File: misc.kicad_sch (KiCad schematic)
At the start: 46 parts, among them J2 Tag-Connect_TC2030-IDC-NL_2x3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, U1 MPFS250T-FCVG484, U2 SDINBDG4-8G, U3 MT25QL01GBBB1EW9-0SIT

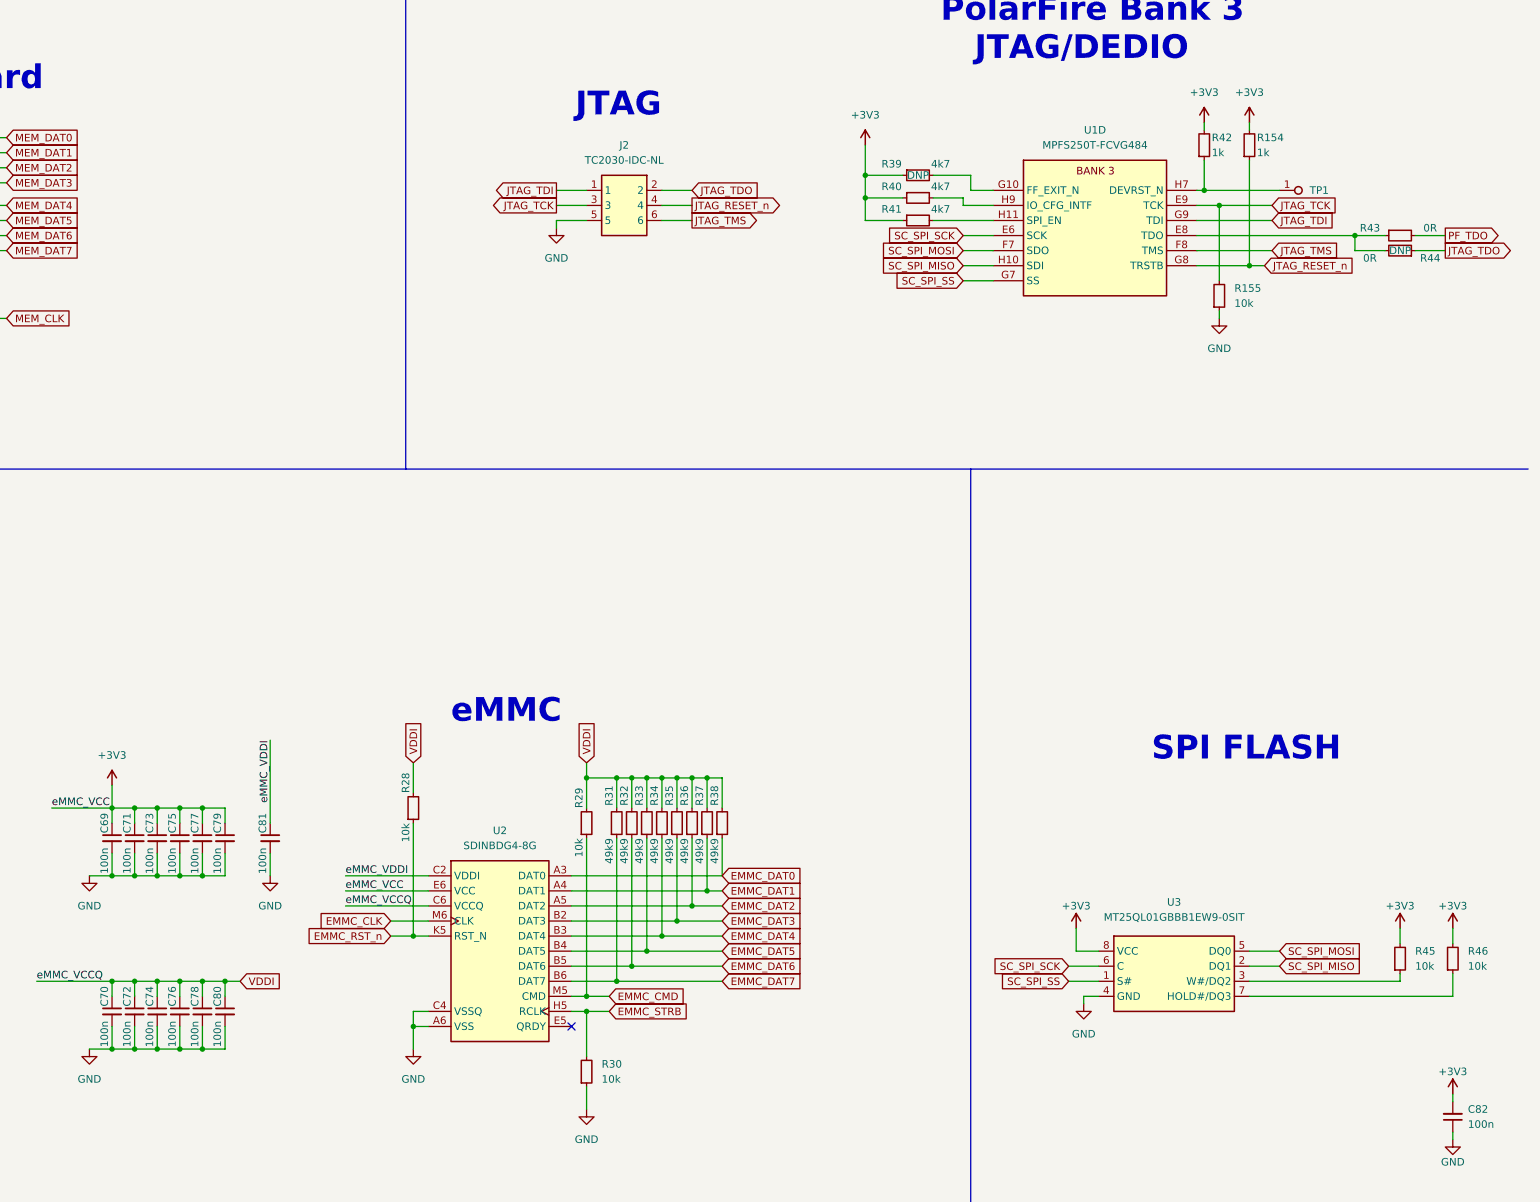
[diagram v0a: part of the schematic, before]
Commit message: [#54899] Update symbols
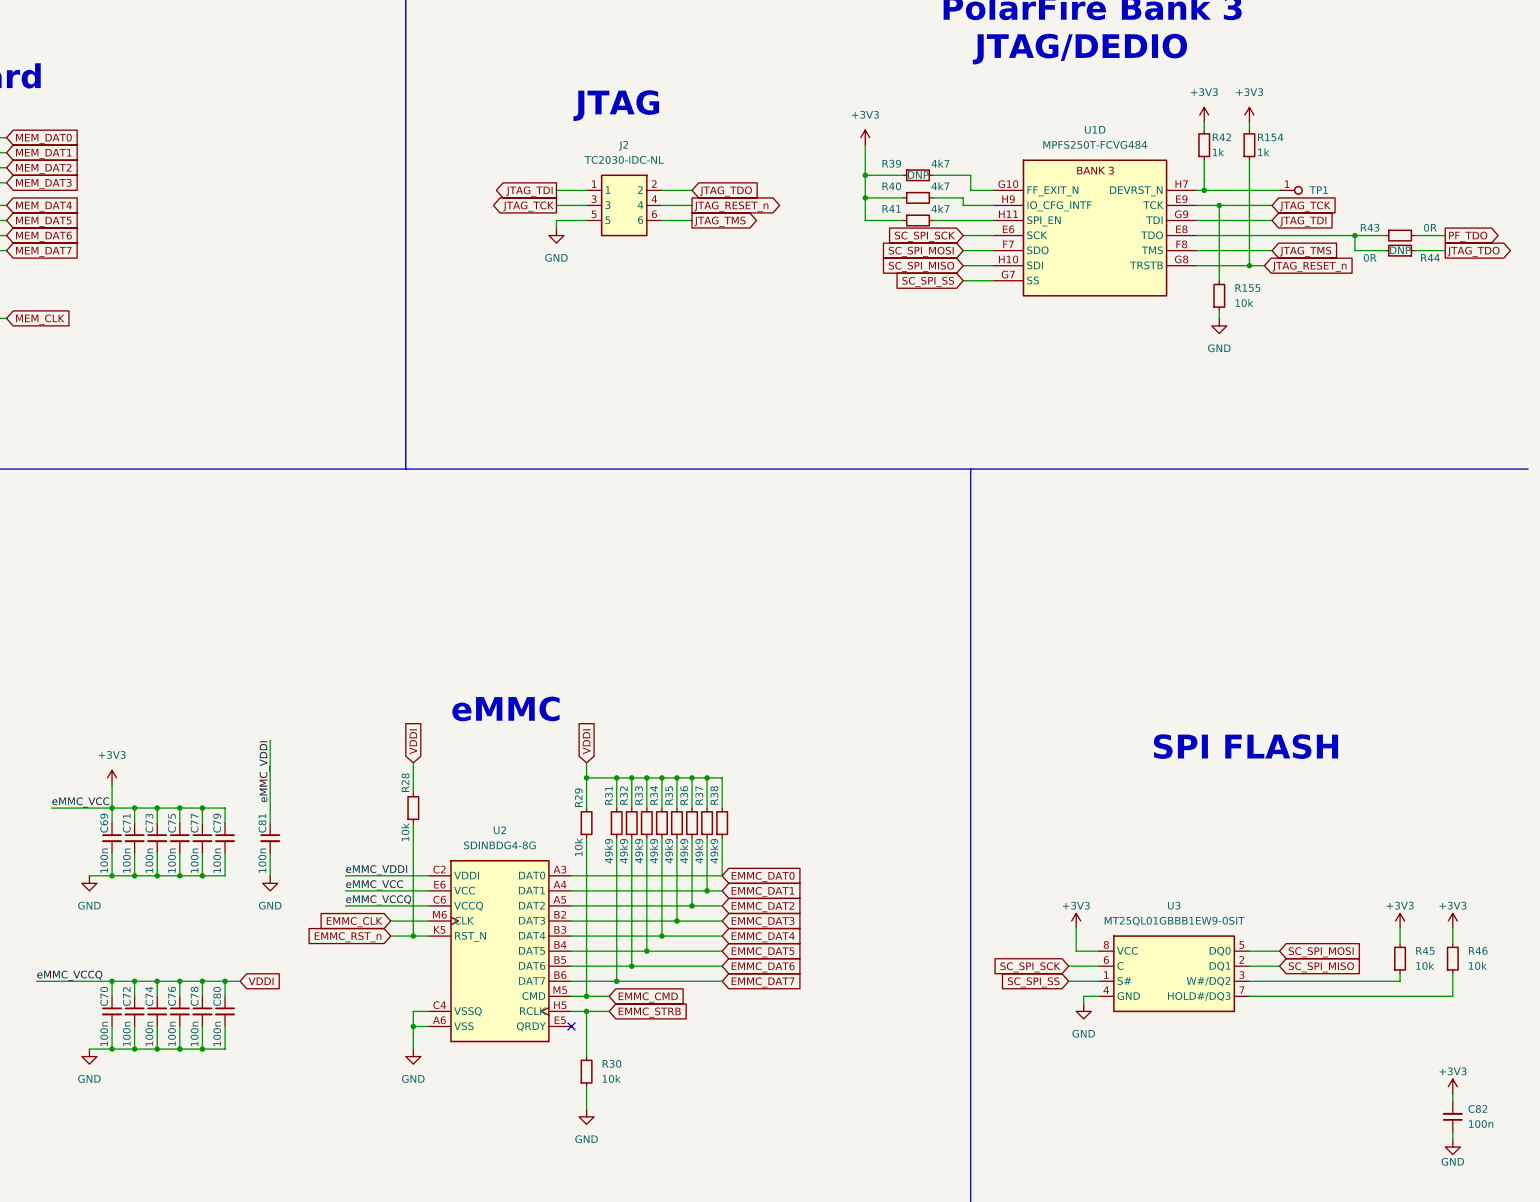
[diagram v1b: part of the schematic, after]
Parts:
- R25, R26, R27, R44: now in the parts list
- U1: footprint antmicro-footprints:BGA-484_19x19mm_Layout22x22_P0.8mm_FCVG484 -> antmicro-footprints:BGA-484_19x19mm_Layout22x22_P0.8mm_MPFS250T-FCVG484
- U3: value MT25QL01GBBB1EW9-0SIT -> MT25QL01GBBB1EW9-0SIT; symbol antmicroMemory:MT25QL01GBBB1EW9-0SIT -> antmicroMemory:MT25QL01GBBB1EW9-0SIT; MPN MT25QL01GBBB1EW9-0SIT -> MT25QL01GBBB1EW9-0SIT
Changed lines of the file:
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@@
   )
   (symbol (lib_id "antmicroResistorNetworksArrays:R_4x0R_0201_array") (at 138.43 66.04 0) (unit 1)
-    (in_bom no) (on_board yes) (dnp no)
+    (in_bom yes) (on_board yes) (dnp no)
     (property "Reference" "R25" (at 143.51 59.69 0)
       (effects (font (size 1.27 1.27) (thickness 0.15)))
@@
   )
   (symbol (lib_id "antmicroResistors0402:R_0R_0402") (at 388.62 85.09 180) (unit 1)
-    (in_bom no) (on_board yes) (dnp no)
+    (in_bom yes) (on_board yes) (dnp no)
     (property "Reference" "R44" (at 391.16 86.36 0)
       (effects (font (size 1.27 1.27) (thickness 0.15)))
@@
   )
   (symbol (lib_id "antmicroResistors0402:R_0R_0402") (at 140.97 96.52 0) (unit 1)
-    (in_bom no) (on_board yes) (dnp no)
+    (in_bom yes) (on_board yes) (dnp no)
     (property "Reference" "R27" (at 138.43 95.25 0)
       (effects (font (size 1.27 1.27) (thickness 0.15)))
@@
       (effects (font (size 1.27 1.27) (thickness 0.15)) (justify left bottom) hide)
     )
-    (property "Footprint" "antmicro-footprints:BGA-484_19x19mm_Layout22x22_P0.8mm_FCVG484" (at 157.48 208.28 0)
+    (property "Footprint" "antmicro-footprints:BGA-484_19x19mm_Layout22x22_P0.8mm_MPFS250T-FCVG484" (at 157.48 208.28 0)
       (effects (font (size 1.27 1.27) (thickness 0.15)) (justify left bottom) hide)
     )
@@
     )
   )
-  (symbol (lib_id "antmicroMemory:MT25QL01GBBB1EW9-0SIT ") (at 335.28 203.2 0) (unit 1)
+  (symbol (lib_id "antmicroMemory:MT25QL01GBBB1EW9-0SIT") (at 335.28 203.2 0) (unit 1)
     (in_bom yes) (on_board yes) (dnp no) (fields_autoplaced)
-    (property "Reference" "U3" (at 347.98 194.945 0)
-      (effects (font (size 1.27 1.27) (thickness 0.15)))
-    )
-    (property "Value" "MT25QL01GBBB1EW9-0SIT " (at 378.46 210.82 0)
+    (property "Reference" "U3" (at 347.98 195.58 0)
+      (effects (font (size 1.27 1.27) (thickness 0.15)))
+    )
+    (property "Value" "MT25QL01GBBB1EW9-0SIT" (at 378.46 210.82 0)
       (effects (font (size 1.27 1.27) (thickness 0.15)) (justify left bottom) hide)
     )
@@
       (effects (font (size 1.27 1.27) (thickness 0.15)) (justify left bottom) hide)
     )
-    (property "Datasheet" "https://www.mouser.pl/datasheet/2/671/mict_s_a0002234966_1-2290738.pdf" (at 378.46 215.9 0)
-      (effects (font (size 1.27 1.27) (thickness 0.15)) (justify left bottom) hide)
-    )
-    (property "MPN" "MT25QL01GBBB1EW9-0SIT " (at 347.98 197.485 0)
+    (property "Datasheet" "https://www.mouser.com/datasheet/2/671/mict_s_a0002234966_1-2290738.pdf" (at 378.46 215.9 0)
+      (effects (font (size 1.27 1.27) (thickness 0.15)) (justify left bottom) hide)
+    )
+    (property "MPN" "MT25QL01GBBB1EW9-0SIT" (at 347.98 198.12 0)
       (effects (font (size 1.27 1.27) (thickness 0.15)))
     )
@@
   )
   (symbol (lib_id "antmicroResistorNetworksArrays:R_4x0R_0201_array") (at 138.43 77.47 0) (unit 1)
-    (in_bom no) (on_board yes) (dnp no)
+    (in_bom yes) (on_board yes) (dnp no)
     (property "Reference" "R26" (at 143.51 87.63 0)
       (effects (font (size 1.27 1.27) (thickness 0.15)))
@@
       (effects (font (size 1.27 1.27) (thickness 0.15)) (justify left bottom) hide)
     )
-    (property "Footprint" "antmicro-footprints:BGA-484_19x19mm_Layout22x22_P0.8mm_FCVG484" (at 421.64 85.09 0)
-      (effects (font (size 1.27 1.27) (thickness 0.15)) (justify left bottom) hide)
-    )
+    (property "Footprint" "antmicro-footprints:BGA-484_19x19mm_Layout22x22_P0.8mm_MPFS250T-FCVG484" (at 421.64 85.09 0)
+      (effects (font (size 1.27 1.27) (thickness 0.15)) (justify left bottom) hide)
+    )
